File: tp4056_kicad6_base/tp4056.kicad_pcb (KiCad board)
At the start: 2 copper layers, 50 x 32 mm, 33 parts, among them J1 USB_B_Micro, J10 Conn_01x02_Male, J2 Conn_01x01_Female, J3 Conn_01x01_Female, J4 Conn_01x01_Female, J5 Conn_01x01_Female, J6 Conn_01x01_Female, J7 Conn_01x01_Female, J8 Conn_01x02_Male, J9 Conn_01x02_Male, Q1 FDN340P, Q2 FS8205A, U1 TP4056, U2 DW01, U3 LM1117-3.3

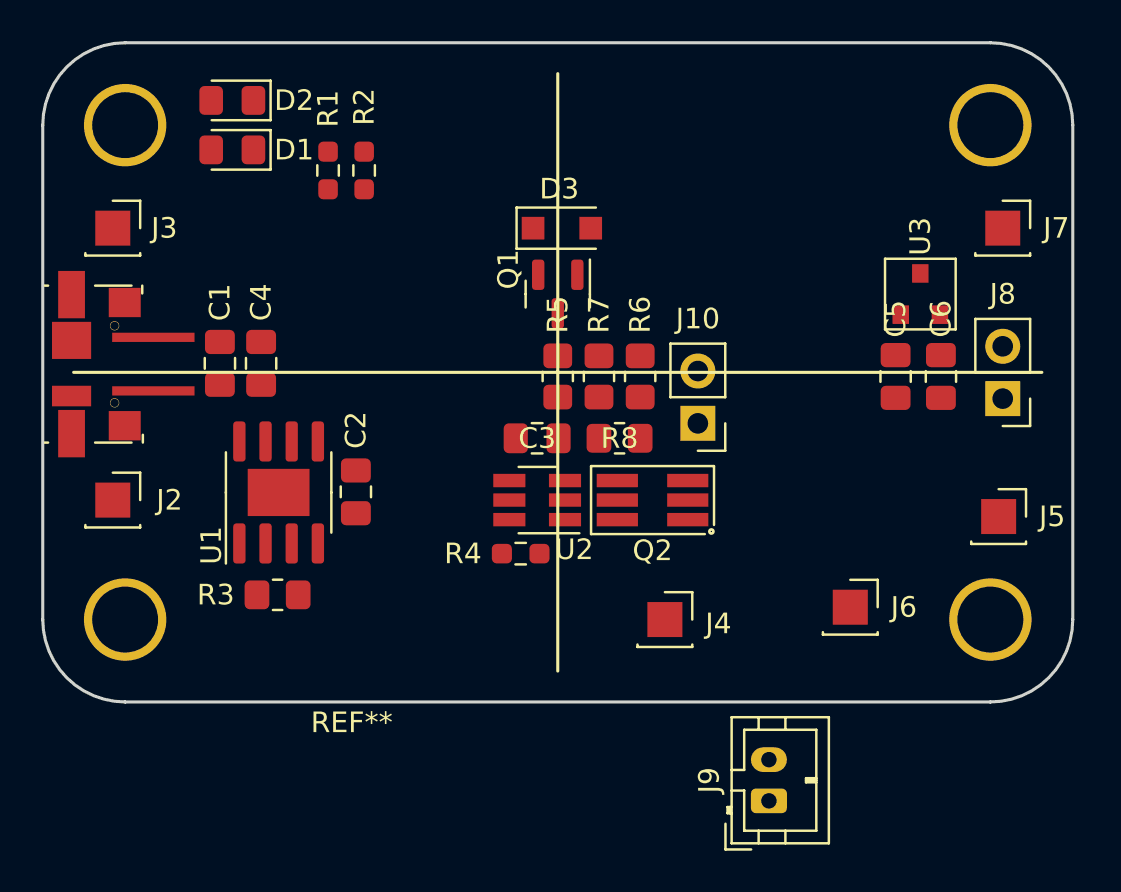
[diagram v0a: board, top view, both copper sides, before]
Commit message: pcb. Board ready in 4032
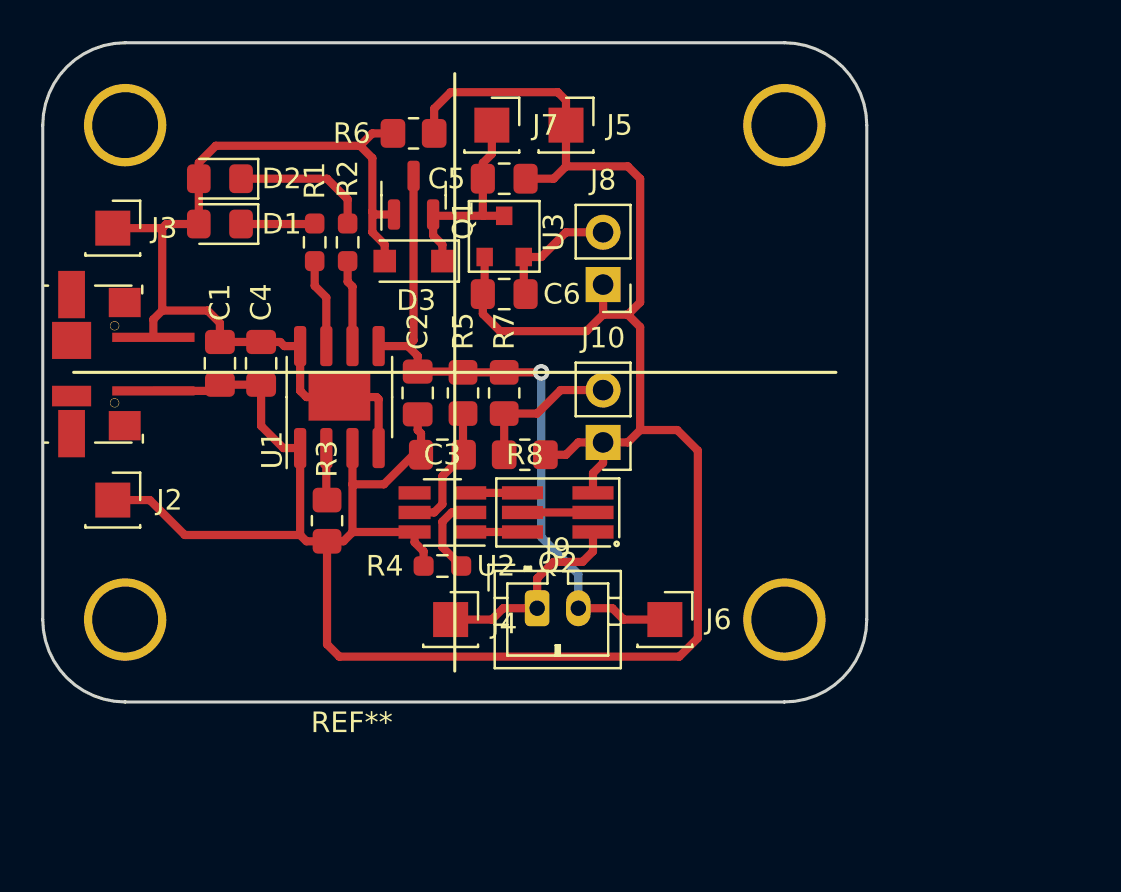
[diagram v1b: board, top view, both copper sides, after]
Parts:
- REF**: value SoBr_5032 -> SoBr_4032; footprint SoBr:SoBr_5032 -> SoBr:SoBr_4032
- moved J5 28.3 mm to (179.8, 92.4)
- moved J7 25.3 mm to (176.2, 92.4)
- moved C6 21.6 mm to (176.8, 100.6), turned to 180 degrees
- moved C5 21.3 mm to (176.8, 95.0), turned to 0 degrees
- moved U3 20.4 mm to (176.8, 97.8)
- moved J8 20.2 mm to (181.6, 100.1)
- moved R6 16.1 mm to (172.4, 92.8), turned to 0 degrees
- moved J9 14.6 mm to (178.4, 115.8), turned to 0 degrees
- moved J4 10.4 mm to (174.2, 116.4)
- moved J6 9.02 mm to (184.6, 116.4)
- moved Q1 8.49 mm to (172.4, 95.8), turned to 90 degrees
- moved D3 7.38 mm to (172.4, 99.0), turned to 180 degrees
- moved C2 5.66 mm to (172.6, 105.4)
- moved U1 5.49 mm to (168.8, 105.6)
- moved J10 4.69 mm to (181.6, 107.8)
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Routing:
- net Earth: track 0.00 -> 127.2 mm
- net VBUS: track 0.00 -> 46.4 mm
- net /BAT+: track 0.00 -> 33.9 mm, vias 0 -> 1
- net /OUT+: track 0.00 -> 10.5 mm
- net /BAT-: track 0.00 -> 10.1 mm
- net /measurment: track 0.00 -> 7.27 mm
- net Net-(D2-Pad1): track 0.00 -> 6.76 mm
- net Net-(C3-Pad1): track 0.00 -> 6.36 mm
- net Net-(C6-Pad1): track 0.00 -> 6.18 mm
- net Net-(U1-Pad7): track 0.00 -> 4.36 mm
- net Net-(U1-Pad6): track 0.00 -> 4.22 mm
- net Net-(R4-Pad2): track 0.00 -> 4.07 mm
- net Net-(D1-Pad1): track 0.00 -> 3.59 mm
- net Net-(Q2-Pad2): track 0.00 -> 3.42 mm
- net Net-(Q2-Pad6): track 0.00 -> 2.54 mm
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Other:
- board size 50 x 32 mm -> 40 x 32 mm
